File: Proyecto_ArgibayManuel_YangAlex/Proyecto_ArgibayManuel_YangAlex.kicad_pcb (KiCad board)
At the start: 2 copper layers, 130.5 x 67.5 mm, 72 parts, among them IC1 LM1117, J1 Conn_01x02, J10 Con_1x2, J11 Con_1x2, J12 Con_ICSP, J2 Conn_01x01, J3 Con_1x2, J4 Con_1x2, J5 Con_1x2, J6 Con_1x2, J7 Conn_01x03, J8 Conn_01x03, J9 Conn_01x03_Pin, K1 RT314012, K2 RT314012, Q1 2N2222, Q2 2N2222, SW1 SW_Push, SW2 SW_Push, SW3 SW_Push, SW4 SW_Push, U1 PIC18F258-I_SO, U2 HDC2010YPAR, U3 LT1716IS5TRMPBF, U4 LT1716IS5TRMPBF, U6 DRV8871DDA, U7 DRV8871DDA, U8 MCP2551-I-P, U9 SN74LVC2T45YZP, X1 DB9, X2 DB9, Y1 Crystal

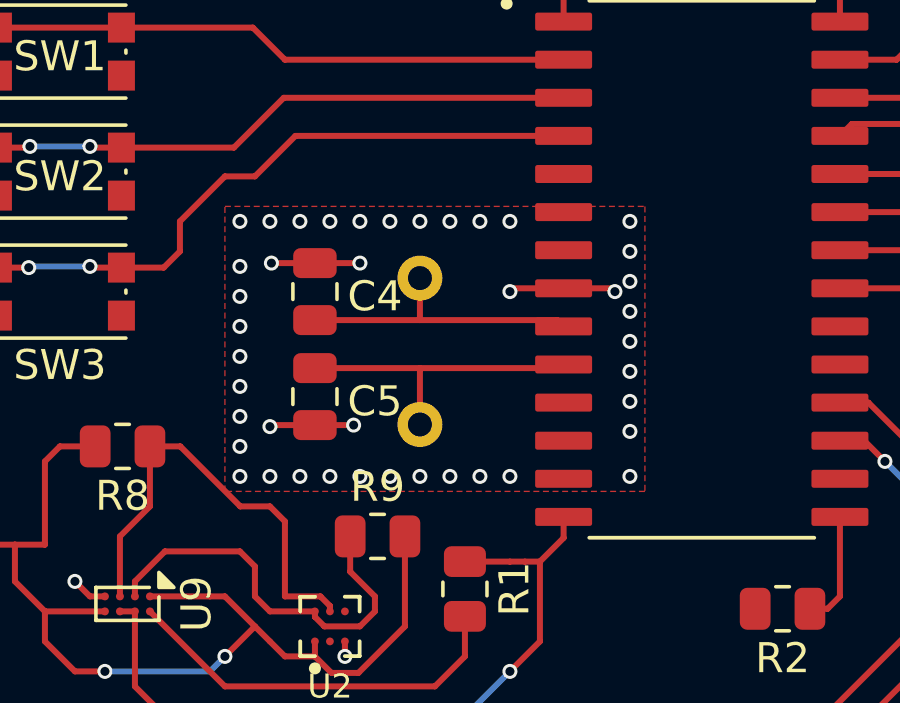
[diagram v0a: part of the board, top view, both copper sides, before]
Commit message: final
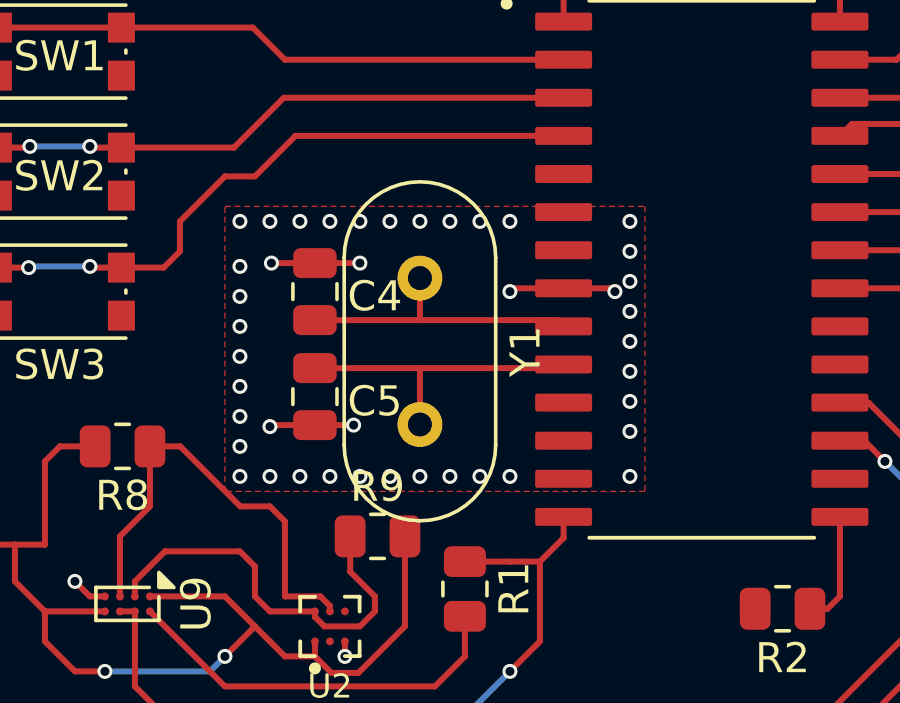
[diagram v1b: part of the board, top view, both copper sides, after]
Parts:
- Y1: moved to F.Cu
